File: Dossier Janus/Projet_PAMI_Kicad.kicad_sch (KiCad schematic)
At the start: 34 parts, among them SW1 SW_Push, U1 LM2596S-3.3, U2 STM32L552CCTx, U4 LM2596S-3.3

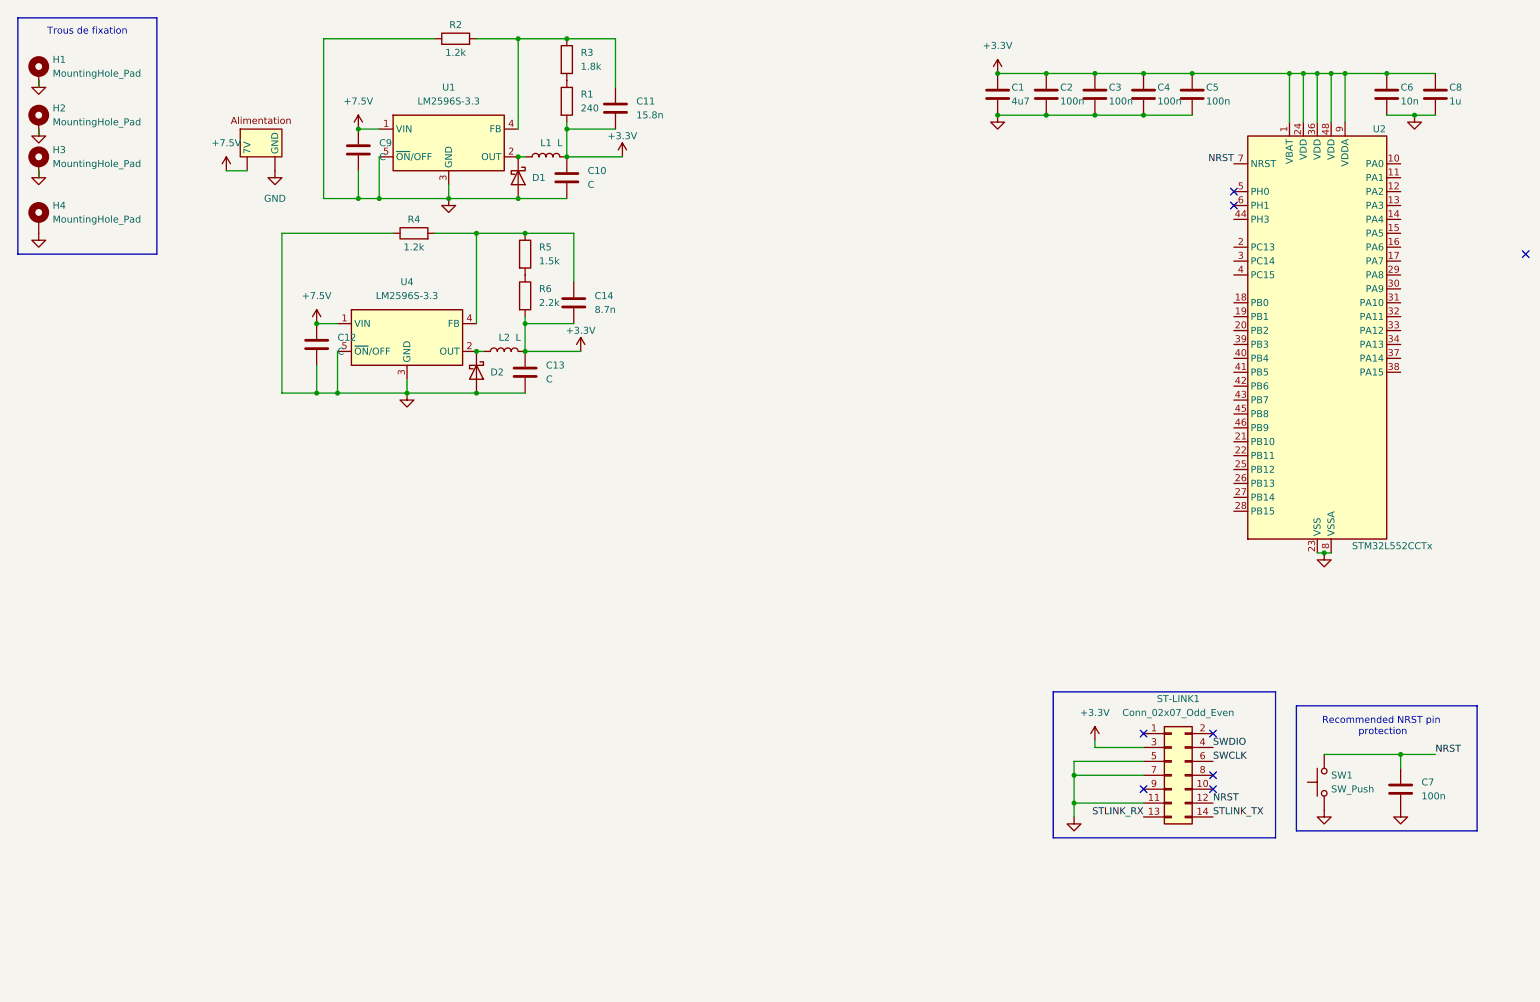
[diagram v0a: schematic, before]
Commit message: Finalisation schematic + ressources
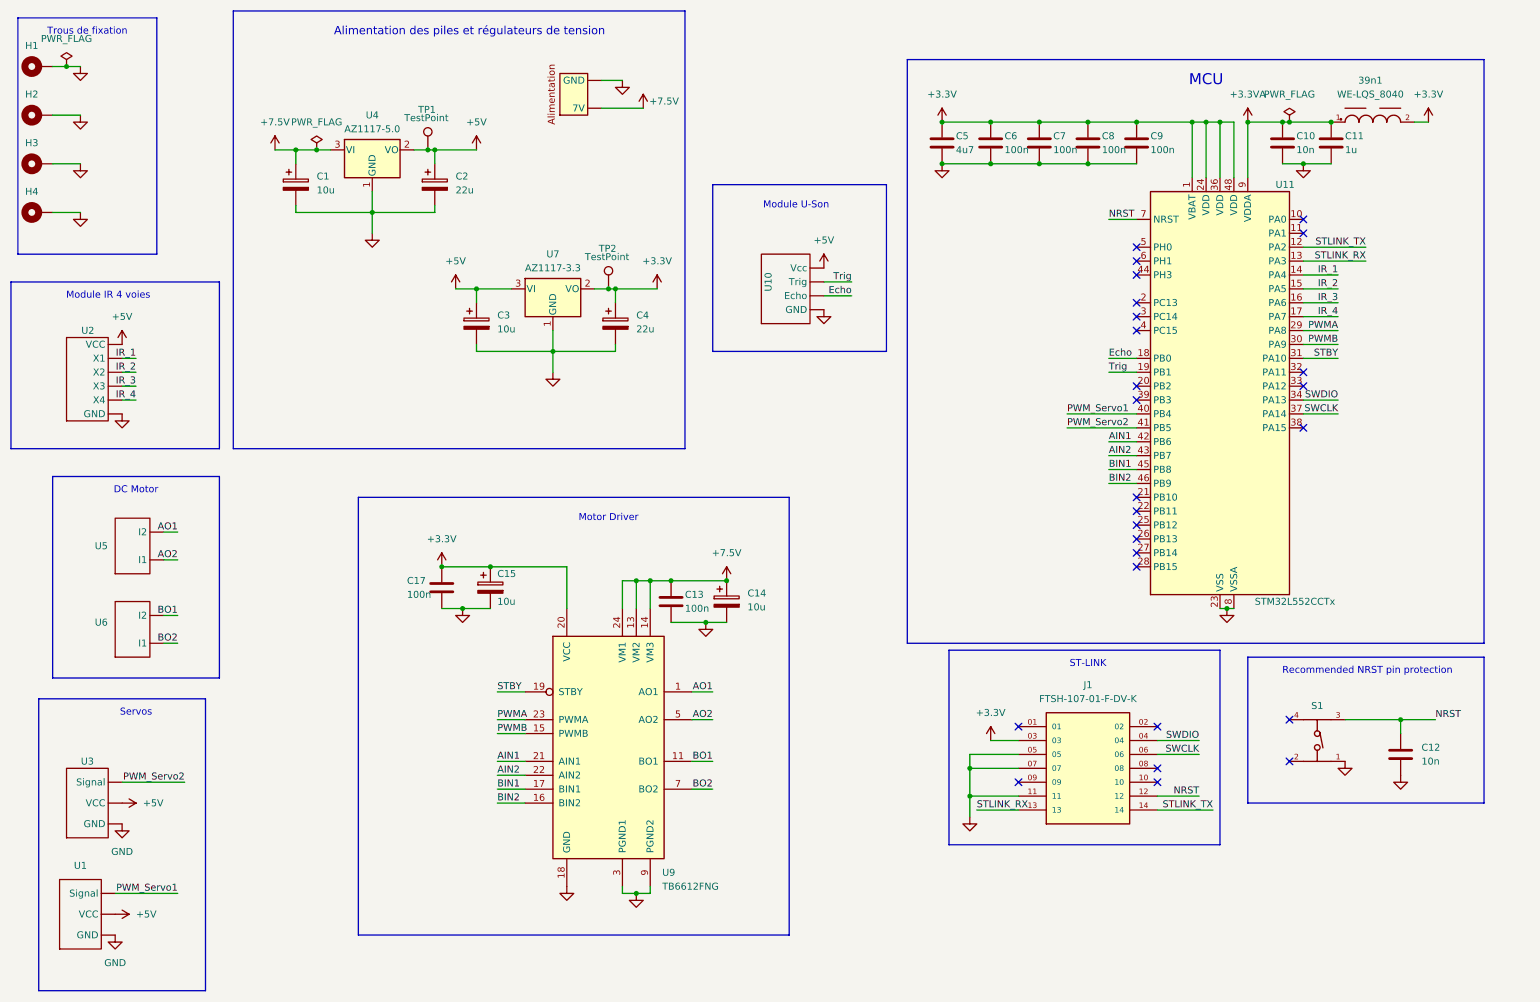
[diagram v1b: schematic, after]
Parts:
- removed C10, C12, C9: C, symbol Device:C
- removed C11: 15.8n, symbol Device:C
- removed C14: 8.7n, symbol Device:C
- removed D1, D2: D_Schottky, symbol Device:D_Schottky
- removed L1, L2: L, symbol Device:L
- removed R1: 240, symbol Device:R
- removed R2, R4: 1.2k, symbol Device:R
- removed R3: 1.8k, symbol Device:R
- removed R5: 1.5k, symbol Device:R
- removed R6: 2.2k, symbol Device:R
- removed ST-LINK1: Conn_02x07_Odd_Even, symbol Connector_Generic:Conn_02x07_Odd_Even
- removed SW1: SW_Push, symbol Switch:SW_Push
- removed U1, U4: LM2596S-3.3, Package_TO_SOT_SMD:TO-263-5_TabPin3, symbol Regulator_Switching:LM2596S-3.3
- added 39n1: WE-LQS_8040, WE-LQS_8040:WE-LQS_8040, symbol WE-LQS_8040:WE-LQS_8040
- added C1, C14, C15, C3: 10u, Capacitor_SMD:C_Elec_4x5.4, symbol Device:C_Polarized
- added C17: 100n, Capacitor_SMD:C_0402_1005Metric_Pad0.74x0.62mm_HandSolder, symbol Device:C
- added C2, C4: 22u, Capacitor_SMD:C_Elec_5x5.4, symbol Device:C_Polarized
- added J1: FTSH-107-01-F-DV-K, FTSH-107-01-F-DV-K:SAMTEC_FTSH-107-01-F-DV-K, symbol FTSH-107-01-F-DV-K:FTSH-107-01-F-DV-K
- added S1: 430471025826, boutonSMD_wurth430471025826:430471025826, symbol boutonSMD_wurth430471025826:430471025826
- added TP1, TP2: TestPoint, TestPoint:TestPoint_Pad_D2.0mm, symbol Connector:TestPoint
- added U1, U3: ~, Connector_PinHeader_2.54mm:PinHeader_1x03_P2.54mm_Vertical, symbol Library_PAMI:Servo_moteur
- added U10: ~, Connector_PinHeader_2.54mm:PinHeader_1x04_P2.54mm_Vertical, symbol Library_PAMI:Module_Uson
- added U2: ~, Connector_PinHeader_2.54mm:PinHeader_1x06_P2.54mm_Vertical, symbol Library_PAMI:IR_Module_4way
- added U4: AZ1117-5.0, Package_TO_SOT_SMD:SOT-223-3_TabPin2, symbol Regulator_Linear:AZ1117-3.3
- added U5, U6: ~, Connector_PinHeader_2.54mm:PinHeader_1x02_P2.54mm_Vertical, symbol Library_PAMI:Moteur_DC
- added U7: AZ1117-3.3, Package_TO_SOT_SMD:SOT-223-3_TabPin2, symbol Regulator_Linear:AZ1117-3.3
- added U9: TB6612FNG, Package_SO:SSOP-24_5.3x8.2mm_P0.65mm, symbol Driver_Motor:TB6612FNG
- C10: renamed from C6; footprint (none) -> Capacitor_SMD:C_0402_1005Metric_Pad0.74x0.62mm_HandSolder
- C11: renamed from C8; footprint (none) -> Capacitor_SMD:C_0402_1005Metric_Pad0.74x0.62mm_HandSolder
- C12: renamed from C7; value 100n -> 10n; footprint (none) -> Capacitor_SMD:C_0402_1005Metric_Pad0.74x0.62mm_HandSolder
- C13: value C -> 100n; footprint (none) -> Capacitor_SMD:C_0402_1005Metric_Pad0.74x0.62mm_HandSolder
- C5: renamed from C1; footprint (none) -> Capacitor_SMD:C_0805_2012Metric_Pad1.18x1.45mm_HandSolder
- C6: renamed from C2; footprint (none) -> Capacitor_SMD:C_0402_1005Metric_Pad0.74x0.62mm_HandSolder
- C7: renamed from C3; footprint (none) -> Capacitor_SMD:C_0402_1005Metric_Pad0.74x0.62mm_HandSolder
- C8: renamed from C4; footprint (none) -> Capacitor_SMD:C_0402_1005Metric_Pad0.74x0.62mm_HandSolder
- C9: renamed from C5; footprint (none) -> Capacitor_SMD:C_0402_1005Metric_Pad0.74x0.62mm_HandSolder
- H1, H2, H3, H4: footprint (none) -> MountingHole:MountingHole_2.7mm_M2.5_Pad
- U8: renamed from U3; footprint (none) -> Connector_PinHeader_2.54mm:PinHeader_1x02_P2.54mm_Vertical
- renumbered U2 to U11
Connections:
- net +3.3V: now also 39n1.2, C15.1, C17.1, C4.1, J1.03, TP2.1, U7.2 (VO), U9.20 (VCC); no longer C10.1, C11.1, U11.9 (VDDA)
- net +7.5V: now also C13.1, C1.1, C14.1, U4.3 (VI), U9.13 (VM2), U9.14 (VM3), U9.24 (VM1)
- net GND: now also C1.2, C14.2, C15.2, C17.2, C2.2, C3.2, C4.2, J1.05, J1.07, J1.11, S1.1, U1. (VCC), U10. (Vcc), U2. (X4), U3. (VCC), U4.1 (GND), U7.1 (GND), U9.10 (PGND2), U9.18 (GND), U9.3 (PGND1), U9.4 (PGND1), U9.9 (PGND2)
- net NRST: now also J1.12, S1.3
- net STLINK_RX: now also U11.13 (PA3), J1.13
- net STLINK_TX: now also U11.12 (PA2), J1.14
- net SWCLK: now also U11.37 (PA14), J1.06
- net SWDIO: now also U11.34 (PA13), J1.04
- net IR_1: now reaches U11.14 (PA4)
- net IR_1: now also U2. (X4)
- net IR_2: now reaches U11.15 (PA5)
- net IR_2: now also U2. (X4)
- net IR_3: now reaches U11.16 (PA6)
- net IR_3: now also U2. (X4)
- net IR_4: now reaches U11.17 (PA7)
- net IR_4: now also U2. (X4)
- net Echo: now reaches U11.18 (PB0)
- net Echo: now also U10. (Vcc)
- net Trig: now reaches U11.19 (PB1)
- net Trig: now also U10. (Vcc)
- net PWMA: now reaches U11.29 (PA8)
- net PWMA: now also U9.23 (PWMA)
- net PWMB: now reaches U11.30 (PA9)
- net PWMB: now also U9.15 (PWMB)
- net STBY: now reaches U11.31 (PA10)
- net STBY: now also U9.19 (STBY)
- net PWM_Servo1: now reaches U11.40 (PB4)
- net PWM_Servo1: now also U1. (VCC)
- net PWM_Servo2: now reaches U11.41 (PB5)
- net PWM_Servo2: now also U3. (VCC)
- net AIN1: now reaches U11.42 (PB6)
- net AIN1: now also U9.21 (AIN1)
- net AIN2: now reaches U11.43 (PB7)
- net AIN2: now also U9.22 (AIN2)
- net BIN1: now reaches U11.45 (PB8)
- net BIN1: now also U9.17 (BIN1)
- net BIN2: now reaches U11.46 (PB9)
- net BIN2: now also U9.16 (BIN2)
- new net +3.3VA: 39n1.1, C10.1, C11.1, U11.9 (VDDA)
- new net +5V: C2.1, C3.1, TP1.1, U1. (VCC), U10. (Vcc), U2. (X4), U3. (VCC), U4.2 (VO), U7.3 (VI)
- new net AO1: U5. (I2), U9.1 (AO1), U9.2 (AO1)
- new net AO2: U5. (I2), U9.5 (AO2), U9.6 (AO2)
- new net BO1: U6. (I2), U9.11 (BO1), U9.12 (BO1)
- new net BO2: U6. (I2), U9.7 (BO2), U9.8 (BO2)
- no-connect marks 8 -> 26
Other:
- note added: "Alimentation des piles et régulateurs de tension"
- note added: "DC Motor"
- note added: "MCU"
- note added: "Module IR 4 voies"
- note added: "Module U-Son"
- note added: "Motor Driver"
- note added: "ST-LINK"
- note added: "Servos"
- moved on the sheet: C10, C11, C12, C5, C6, C7, C8, C9, H1, U11
